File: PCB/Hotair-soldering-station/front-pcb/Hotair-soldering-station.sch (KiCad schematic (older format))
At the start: 54 parts, among them J1 fan_reg_pot, J2 main-board-conn, J3 hot_on, J4 solder_on, Q1 BC817, Q10 BC807, Q11 BC807, Q12 BC807, Q13 BC807, Q14 BC807, Q2 BC817, Q3 BC817, Q4 BC817, Q5 BC817, Q6 BC817, Q7 BC817, Q8 BC817, Q9 BC807, SW1 HOTAIR_UP, SW2 HOTAIR_DOWN, SW3 SIRON_UP, SW4 SIRON_DOWN, U1 74HC595D, U2 74HC595D, U3 My-Footprints:3-digit-7-segme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, U4 3-dig-7-seg-display-common-an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

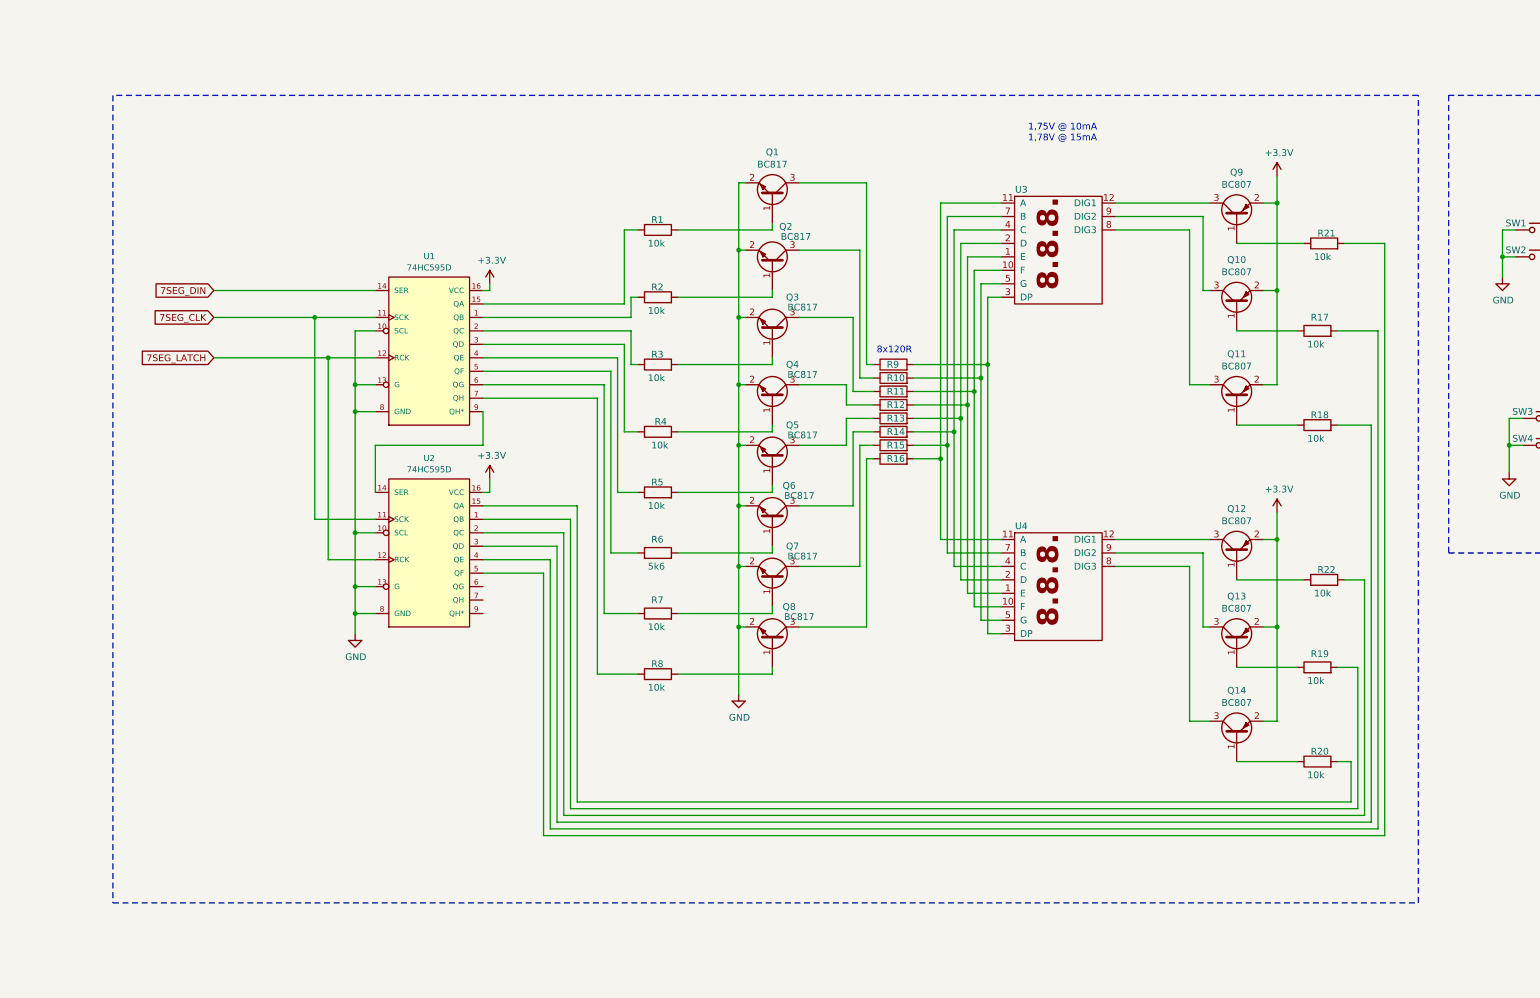
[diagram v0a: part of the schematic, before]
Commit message: routing progress
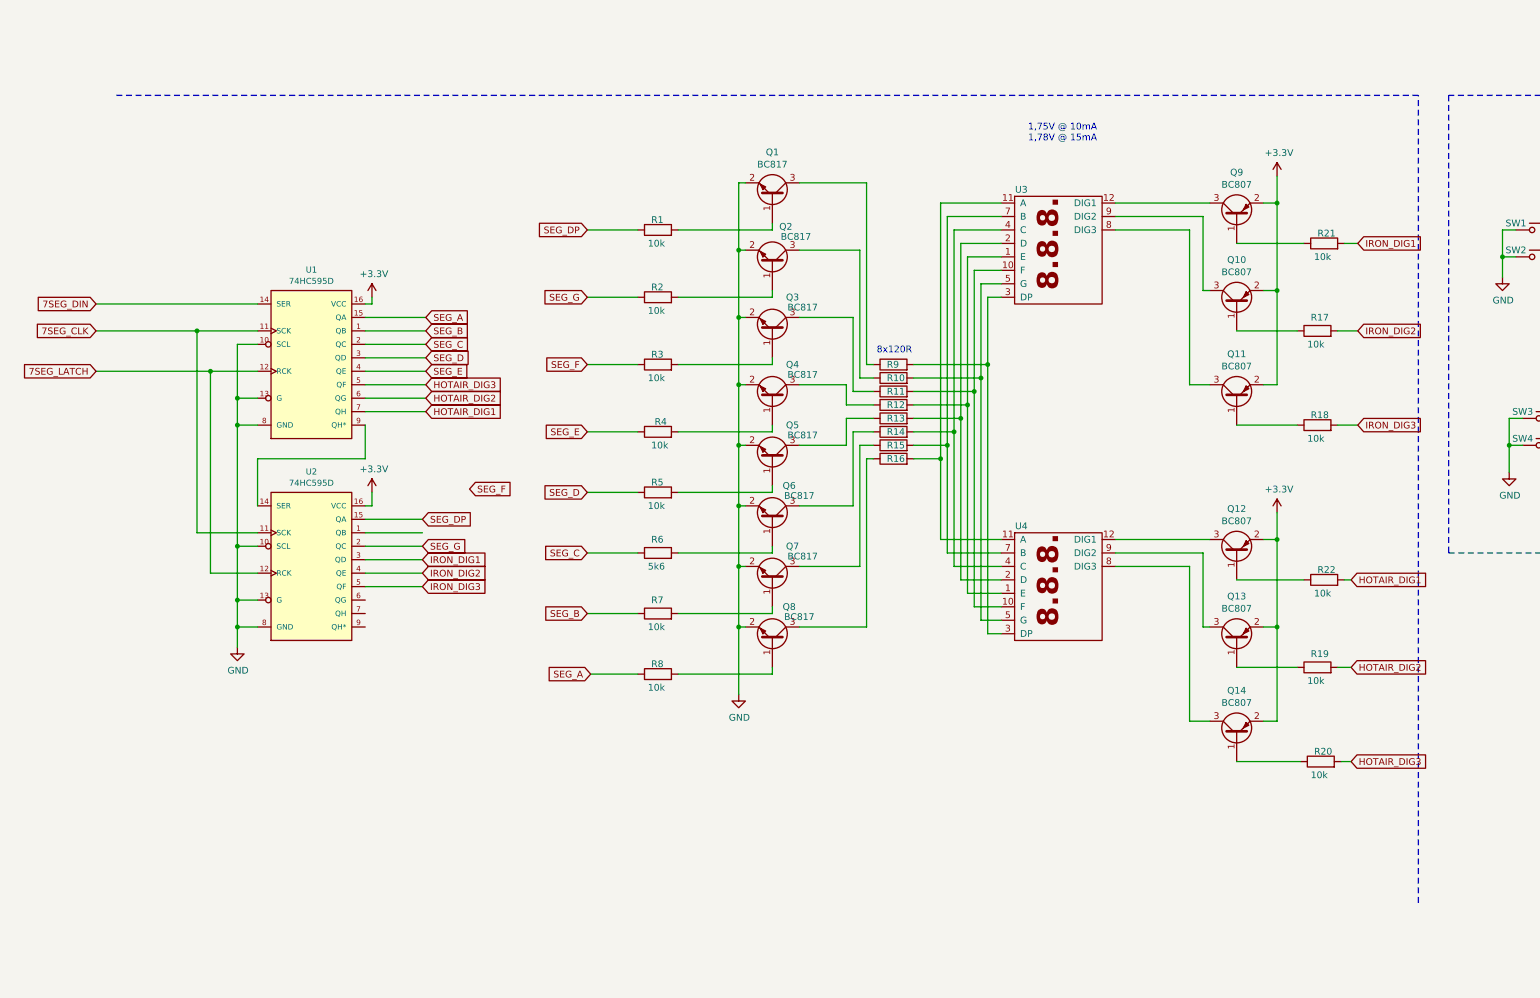
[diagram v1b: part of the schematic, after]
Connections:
- net SEG_B: now reaches U1.1 (QB)
- net SEG_B: now also R7.1; no longer R2.1
- net SEG_A: now reaches U1.15 (QA)
- net SEG_A: now also R8.1; no longer R1.1
- net SEG_C: now reaches U1.2 (QC)
- net SEG_C: now also R6.1; no longer R3.1
- net SEG_D: now reaches U1.3 (QD)
- net SEG_D: now also R5.1; no longer R4.1
- net SEG_E: now reaches U1.4 (QE)
- net SEG_E: now also R4.1; no longer R5.1
- net HOTAIR_DIG3: now reaches U1.5 (QF)
- net HOTAIR_DIG3: now also R20.2; no longer R6.1
- net HOTAIR_DIG2: now reaches U1.6 (QG)
- net HOTAIR_DIG2: now also R19.2; no longer R7.1
- net HOTAIR_DIG1: now reaches U1.7 (QH)
- net HOTAIR_DIG1: now also R22.2; no longer R8.1
- net at U2.1 (QB): no longer R19.2
- net SEG_DP: now reaches U2.15 (QA)
- net SEG_DP: now also R1.1; no longer R20.2
- net SEG_G: now reaches U2.2 (QC)
- net SEG_G: now also R2.1; no longer R22.2
- net IRON_DIG1: now reaches U2.3 (QD)
- net IRON_DIG1: now also R21.2; no longer R18.2
- net IRON_DIG2: now reaches R17.2, U2.4 (QE)
- net IRON_DIG3: now reaches U2.5 (QF)
- net IRON_DIG3: now also R18.2; no longer R21.2
- new net SEG_F: R3.1
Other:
- moved on the sheet: R20, U1, U2
